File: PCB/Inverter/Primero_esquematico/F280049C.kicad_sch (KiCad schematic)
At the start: 1 part, among them U21 F280049CPZS

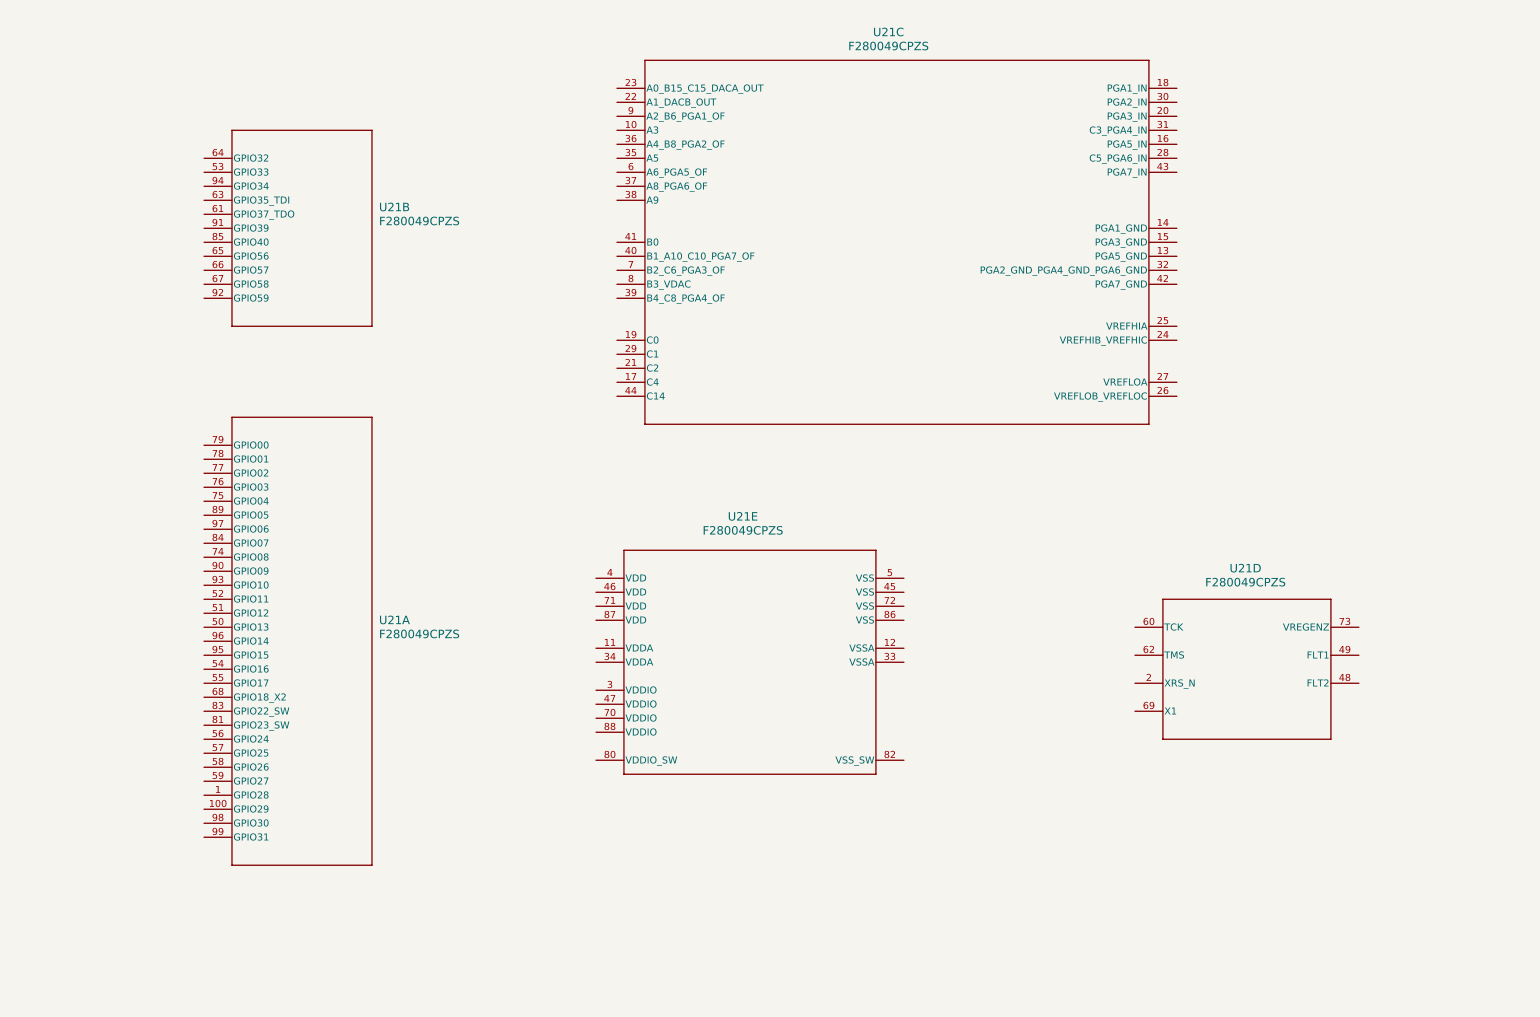
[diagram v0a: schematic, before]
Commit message: Esquematico practicamente terminado
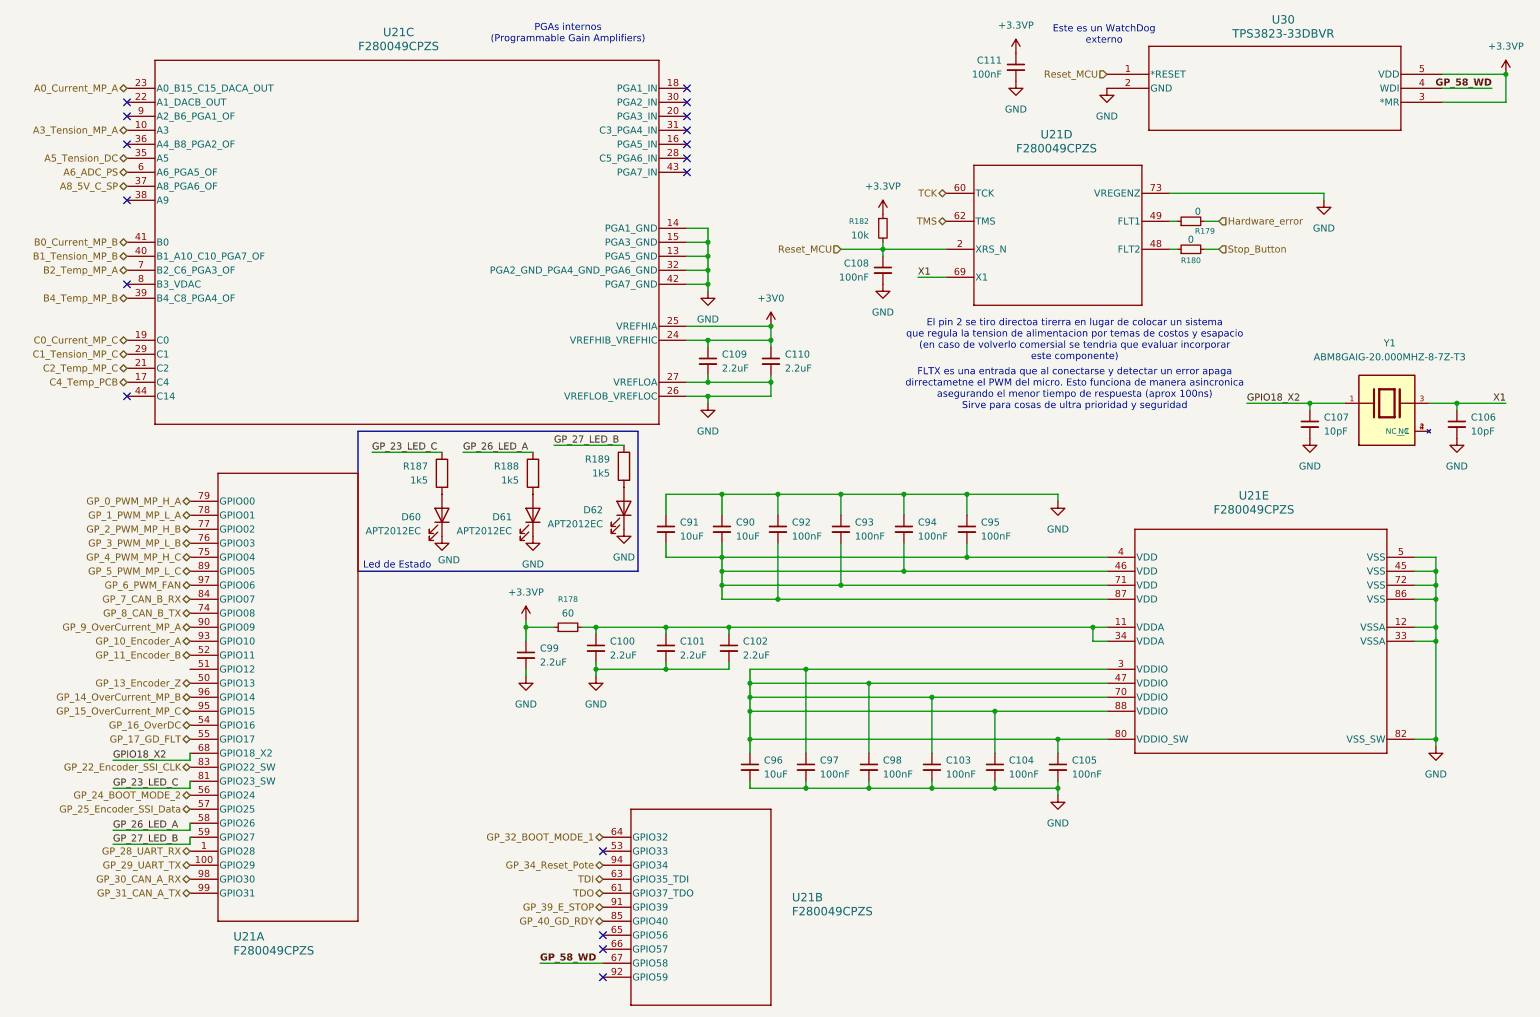
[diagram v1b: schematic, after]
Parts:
- added C100, C101, C102, C109, C110, C99: 2.2uF, Capacitor_SMD:C_0603_1608Metric, symbol Device:C_Small
- added C103, C104, C105, C108, C111, C92, C93, C94, C95, C97, C98: 100nF, Capacitor_SMD:C_0603_1608Metric, symbol Device:C_Small
- added C106, C107: 10pF, Capacitor_SMD:C_0402_1005Metric, symbol Device:C_Small
- added C90, C91, C96: 10uF, Capacitor_SMD:C_0805_2012Metric, symbol Device:C_Small
- added D60, D61, D62: APT2012EC, LED_SMD:LED_0805_2012Metric, symbol Device:LED
- added R178: 60, Resistor_SMD:R_0402_1005Metric, symbol Device:R_Small
- added R179, R180: 0, Resistor_SMD:R_0402_1005Metric, symbol Device:R_Small
- added R182: 10k, Resistor_SMD:R_0402_1005Metric, symbol Device:R_Small
- added R187, R188, R189: 1k5, Resistor_SMD:R_0402_1005Metric, symbol Device:R
- added U30: TPS3823-33DBVR, Snapeda:DBV5-L, symbol Snapeda:TPS3823-33DBVR
- added Y1: ABM8GAIG-20.000MHZ-8-7Z-T3, Snapeda:XTAL_ABM8GAIG-20.000MHZ-8-7Z-T3, symbol Snapeda:ABM8GAIG-20.000MHZ-8-7Z-T3
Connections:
- net GP_28_UART_RX: now reaches U21.1 (GPIO28)
- net GP_29_UART_TX: now reaches U21.100 (GPIO29)
- net GP_13_Encoder_Z: now reaches U21.50 (GPIO13)
- net GP_11_Encoder_B: now reaches U21.52 (GPIO11)
- net GP_16_OverDC: now reaches U21.54 (GPIO16)
- net GP_17_GD_FLT: now reaches U21.55 (GPIO17)
- net GP_24_BOOT_MODE_2: now reaches U21.56 (GPIO24)
- net GP_25_Encoder_SSI_Data: now reaches U21.57 (GPIO25)
- net GP_26_LED_A: now reaches U21.58 (GPIO26)
- net GP_26_LED_A: now also R188.1
- net GP_27_LED_B: now reaches U21.59 (GPIO27)
- net GP_27_LED_B: now also R189.1
- net GPIO18_X2: now reaches U21.68 (GPIO18_X2)
- net GPIO18_X2: now also C107.1, Y1.1
- net GP_8_CAN_B_TX: now reaches U21.74 (GPIO08)
- net GP_4_PWM_MP_H_C: now reaches U21.75 (GPIO04)
- net GP_3_PWM_MP_L_B: now reaches U21.76 (GPIO03)
- net GP_2_PWM_MP_H_B: now reaches U21.77 (GPIO02)
- net GP_1_PWM_MP_L_A: now reaches U21.78 (GPIO01)
- net GP_0_PWM_MP_H_A: now reaches U21.79 (GPIO00)
- net GP_23_LED_C: now reaches U21.81 (GPIO23_SW)
- net GP_23_LED_C: now also R187.1
- net GP_22_Encoder_SSI_CLK: now reaches U21.83 (GPIO22_SW)
- net GP_7_CAN_B_RX: now reaches U21.84 (GPIO07)
- net GP_5_PWM_MP_L_C: now reaches U21.89 (GPIO05)
- net GP_9_OverCurrent_MP_A: now reaches U21.90 (GPIO09)
- net GP_10_Encoder_A: now reaches U21.93 (GPIO10)
- net GP_15_OverCurrent_MP_C: now reaches U21.95 (GPIO15)
- net GP_14_OverCurrent_MP_B: now reaches U21.96 (GPIO14)
- net GP_6_PWM_FAN: now reaches U21.97 (GPIO06)
- net GP_30_CAN_A_RX: now reaches U21.98 (GPIO30)
- net GP_31_CAN_A_TX: now reaches U21.99 (GPIO31)
- net TDO: now reaches U21.61 (GPIO37_TDO)
- net TDI: now reaches U21.63 (GPIO35_TDI)
- net GP_32_BOOT_MODE_1: now reaches U21.64 (GPIO32)
- net GP_58_WD: now reaches U21.67 (GPIO58)
- net GP_58_WD: now also U30.4 (WDI)
- net GP_40_GD_RDY: now reaches U21.85 (GPIO40)
- net GP_39_E_STOP: now reaches U21.91 (GPIO39)
- net GP_34_Reset_Pote: now reaches U21.94 (GPIO34)
- net Reset_MCU: now reaches U21.2 (XRS_N)
- net Reset_MCU: now also C108.1, R182.2, U30.1 (*RESET)
- net at U21.48 (FLT2): now also R180.1
- net at U21.49 (FLT1): now also R179.1
- net TCK: now reaches U21.60 (TCK)
- net TMS: now reaches U21.62 (TMS)
- net X1: now reaches U21.69 (X1)
- net X1: now also C106.1, Y1.3
- net GND: now reaches U21.73 (VREGENZ)
- net GND: now also U21.12 (VSSA), U21.13 (PGA5_GND), U21.14 (PGA1_GND), U21.15 (PGA3_GND), U21.26 (VREFLOB_VREFLOC), U21.27 (VREFLOA), U21.32 (PGA2_GND_PGA4_GND_PGA6_GND), U21.33 (VSSA), U21.42 (PGA7_GND), U21.45 (VSS), U21.5 (VSS), U21.72 (VSS), U21.82 (VSS_SW), U21.86 (VSS), C100.2, C101.2, C102.2, C103.2, C104.2, C105.2, C106.2, C107.2, C108.2, C109.2, C110.2, C111.2, C90.1, C91.1, C92.1, C93.1, C94.1, C95.1, C96.2, C97.2, C98.2, C99.2, D60.1 (K), D61.1 (K), D62.1 (K), U30.2 (GND)
- net A3_Tension_MP_A: now reaches U21.10 (A3)
- net C4_Temp_PCB: now reaches U21.17 (C4)
- net C0_Current_MP_C: now reaches U21.19 (C0)
- net C2_Temp_MP_C: now reaches U21.21 (C2)
- net A0_Current_MP_A: now reaches U21.23 (A0_B15_C15_DACA_OUT)
- net +3V0: now reaches U21.24 (VREFHIB_VREFHIC)
- net +3V0: now also U21.25 (VREFHIA), C109.1, C110.1
- net C1_Tension_MP_C: now reaches U21.29 (C1)
- net A5_Tension_DC: now reaches U21.35 (A5)
- net A8_5V_C_SP: now reaches U21.37 (A8_PGA6_OF)
- net B4_Temp_MP_B: now reaches U21.39 (B4_C8_PGA4_OF)
- net B1_Tension_MP_B: now reaches U21.40 (B1_A10_C10_PGA7_OF)
- net B0_Current_MP_B: now reaches U21.41 (B0)
- net A6_ADC_PS: now reaches U21.6 (A6_PGA5_OF)
- net B2_Temp_MP_A: now reaches U21.7 (B2_C6_PGA3_OF)
- net at U21.11 (VDDA): now also U21.34 (VDDA), C100.1, C101.1, C102.1, R178.2
- net at U21.3 (VDDIO): now also U21.47 (VDDIO), U21.70 (VDDIO), U21.80 (VDDIO_SW), U21.88 (VDDIO), C103.1, C104.1, C105.1, C96.1, C97.1, C98.1
- net at U21.4 (VDD): now also U21.46 (VDD), U21.71 (VDD), U21.87 (VDD), C90.2, C91.2, C92.2, C93.2, C94.2, C95.2
- new net: Y1.2 (NC), Y1.4 (NC__1)
- new net: D61.2 (A), R188.2
- new net: D60.2 (A), R187.2
- new net: D62.2 (A), R189.2
- new net +3.3VP: C111.1, C99.1, R178.1, R182.1, U30.3 (*MR), U30.5 (VDD)
- new net Hardware_error: R179.2
- new net Stop_Button: R180.2
- no-connect marks 0 -> 17
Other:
- note added: "El pin 2 se tiro directoa tirerra en lugar de colocar un sistema que regula la tension de alimentacion por temas de costos y esapacio (en caso de volverlo comersial se tendria que evaluar incorporar este componente)"
- note added: "Este es un WatchDog externo"
- note added: "FLTX es una entrada que al conectarse y detectar un error apaga dirrectametne el PWM del micro. Esto funciona de manera asincronica asegurando el menor tiempo de respuesta (aprox 100ns) Sirve para cosas de ultra prioridad y seguridad"
- note added: "Led de Estado"
- note added: "PGAs internos (Programmable Gain Amplifiers)"
- moved on the sheet: U21A, U21B, U21C, U21D, U21E
